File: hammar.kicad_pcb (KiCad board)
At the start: 2 copper layers, 97.5 x 55 mm, 118 parts, among them J1 8x screw terminal, 5,08mm spa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, J10 1x2, J11 1x4, J12 1x3, J13 1x8, J14 1x3, J15 1x3, J16 1x3, J2 Micro_SD_Holder, J3 USB_C_Receptacle_USB2.0, J4 1x4, J5 1x4, J6 1x4, J7 1x4, J8 1x4, J9 1x2, Q1 S9014 or equivalent, Q2 S9014 or equivalent, Q3 TI CSD17310Q5A or equivalent, Q4 PMV40UN2R or equivalent, Q5 PMV40UN2R or equivalent, SW1 SW_MEC_5G, U1 A4988, U2 A4988, U3 A4988, U4 A4988, U5 DPAK 3,3v linear regulator + 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, U6 ESP32-WROOM-32E, U7 CH340G, Y1 Resonator_12mhz

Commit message: updated bom++
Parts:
- D6: value USB protection diode, >500mA 24V -> USB protection diode, >500mA >24V. Silicon fine
- F1: value 25A Mini fuse + Keystone 3557 fuse holders, or equivalent -> 15A Mini fuse + Keystone 3557 fuse holders, or equivalent
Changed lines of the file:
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@@
       (effects (font (size 1 1) (thickness 0.15)))
     )
-    (fp_text value "USB protection diode, >500mA 24V" (at -0.25 2.25) (layer "F.Fab")
+    (fp_text value "USB protection diode, >500mA >24V. Silicon fine" (at -0.25 2.25) (layer "F.Fab")
       (effects (font (size 1 1) (thickness 0.15)))
     )
@@
       (effects (font (size 1 1) (thickness 0.15)))
     )
-    (fp_text value "25A Mini fuse + Keystone 3557 fuse holders, or equivalent" (at 0 -4 -90 unlocked) (layer "F.Fab")
-      (effects (font (size 1 1) (thickness 0.15)))
-    )
+    (fp_text value "15A Mini fuse + Keystone 3557 fuse holders, or equivalent" (at 0 -4 -90 unlocked) (layer "F.Fab")
+      (effects (font (size 1 1) (thickness 0.15)))
+    )

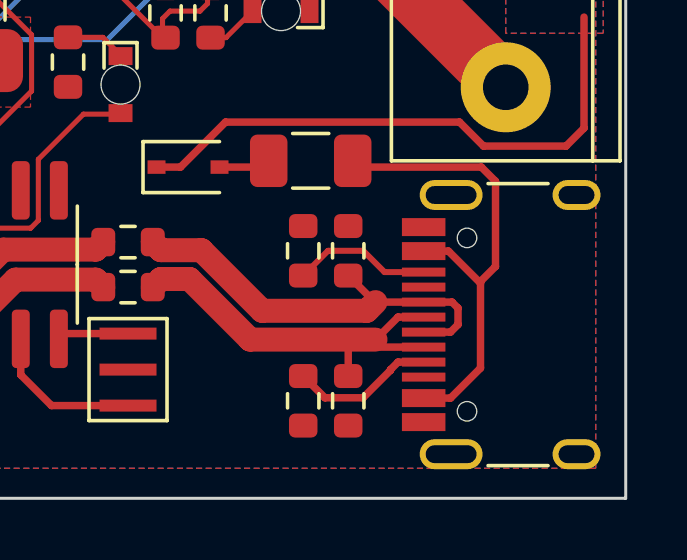
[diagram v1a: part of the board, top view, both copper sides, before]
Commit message: slight reference update
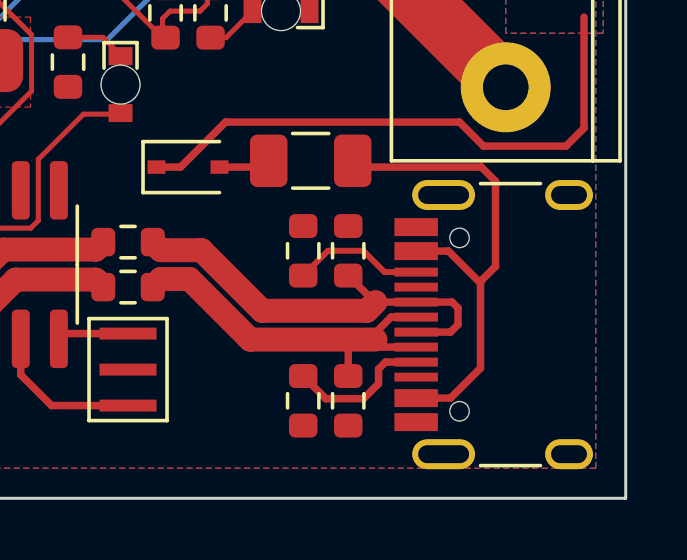
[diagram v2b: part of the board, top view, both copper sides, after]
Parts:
- moved J3 0.25 mm to (185.6, 115.0)
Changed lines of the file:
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@@
   )
   (footprint "Connector_USB:USB_C_Receptacle_HRO_TYPE-C-31-M-12" (layer "F.Cu")
-    (at 185.865 114.972756 90)
+    (at 185.615 114.972756 90)
     (descr "USB Type-C receptacle for USB 2.0 and PD, http://www.krhro.com/uploads/soft/180320/1-1P320120243.pdf")
     (tags "usb usb-c 2.0 pd")
@@
   (segment (start 117.305 93.80897) (end 117.305 93.512874) (width 0.17) (layer "F.Cu") (net 28))
   (segment (start 121.202709 97.460465) (end 118.6503 100.012874) (width 0.17) (layer "F.Cu") (net 28))
-  (segment (start 180.715 116.472756) (end 180.965 116.222756) (width 0.25) (layer "F.Cu") (net 29))
-  (segment (start 177.805 116.687874) (end 178.53 117.412874) (width 0.25) (layer "F.Cu") (net 29))
-  (segment (start 178.53 117.412874) (end 179.797462 117.412874) (width 0.25) (layer "F.Cu") (net 29))
-  (segment (start 180.965 116.222756) (end 181.82 116.222756) (width 0.25) (layer "F.Cu") (net 29))
-  (segment (start 179.797462 117.412874) (end 180.715 116.495336) (width 0.25) (layer "F.Cu") (net 29))
-  (segment (start 180.715 116.495336) (end 180.715 116.472756) (width 0.25) (layer "F.Cu") (net 29))
+  (segment (start 179.815 117.442756) (end 180.315 116.942756) (width 0.25) (layer "F.Cu") (net 29))
+  (segment (start 178.559882 117.442756) (end 179.815 117.442756) (width 0.25) (layer "F.Cu") (net 29))
+  (segment (start 180.545 116.222756) (end 181.82 116.222756) (width 0.25) (layer "F.Cu") (net 29))
+  (segment (start 180.315 116.452756) (end 180.545 116.222756) (width 0.25) (layer "F.Cu") (net 29))
+  (segment (start 177.805 116.687874) (end 178.559882 117.442756) (width 0.25) (layer "F.Cu") (net 29))
+  (segment (start 180.315 116.942756) (end 180.315 116.452756) (width 0.25) (layer "F.Cu") (net 29))
   (segment (start 179.805 112.512874) (end 180.514882 113.222756) (width 0.2) (layer "F.Cu") (net 31))
   (segment (start 177.805 113.337874) (end 178.63 112.512874) (width 0.2) (layer "F.Cu") (net 31))
@@
   (segment (start 176.036176 115.472756) (end 180.215 115.472756) (width 0.8) (layer "F.Cu") (net 48))
   (segment (start 179.305 115.722756) (end 181.82 115.722756) (width 0.25) (layer "F.Cu") (net 48))
+  (segment (start 180.735 114.722756) (end 180.215 115.242756) (width 0.25) (layer "F.Cu") (net 48))
+  (segment (start 181.82 114.722756) (end 180.735 114.722756) (width 0.25) (layer "F.Cu") (net 48))
   (segment (start 172.79 113.722756) (end 173.06 113.452756) (width 0.8) (layer "F.Cu") (net 48))
-  (segment (start 180.965 114.722756) (end 180.215 115.472756) (width 0.25) (layer "F.Cu") (net 48))
+  (segment (start 180.215 115.242756) (end 180.215 115.472756) (width 0.25) (layer "F.Cu") (net 48))
   (segment (start 173.06 113.452756) (end 174.016176 113.452756) (width 0.8) (layer "F.Cu") (net 48))
   (segment (start 174.016176 113.452756) (end 176.036176 115.472756) (width 0.8) (layer "F.Cu") (net 48))
-  (segment (start 181.82 114.722756) (end 180.965 114.722756) (width 0.25) (layer "F.Cu") (net 48))
   (segment (start 179.305 116.687874) (end 179.305 115.722756) (width 0.25) (layer "F.Cu") (net 48))
   (segment (start 106.045 100.907756) (end 106.045 102.907756) (width 0.17) (layer "F.Cu") (net 49))
